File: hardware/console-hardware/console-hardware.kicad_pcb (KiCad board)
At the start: 2 copper layers, 45.7 x 64.8 mm, 42 parts, among them J1 USB_B_Micro, J2 LiPo battery, J3 Conn_01x04, J4 ICSP, J5 Conn_01x20, SW1 SW_Push, SW2 SW_Push, SW3 SW_Push, SW4 SW_Push, SW5 SW_Push, SW6 SW_Push, U1 ATmega32U4-A, U2 MCP73831-2-OT, U3 MIC5219-3.3YM5, X1 16 MHz

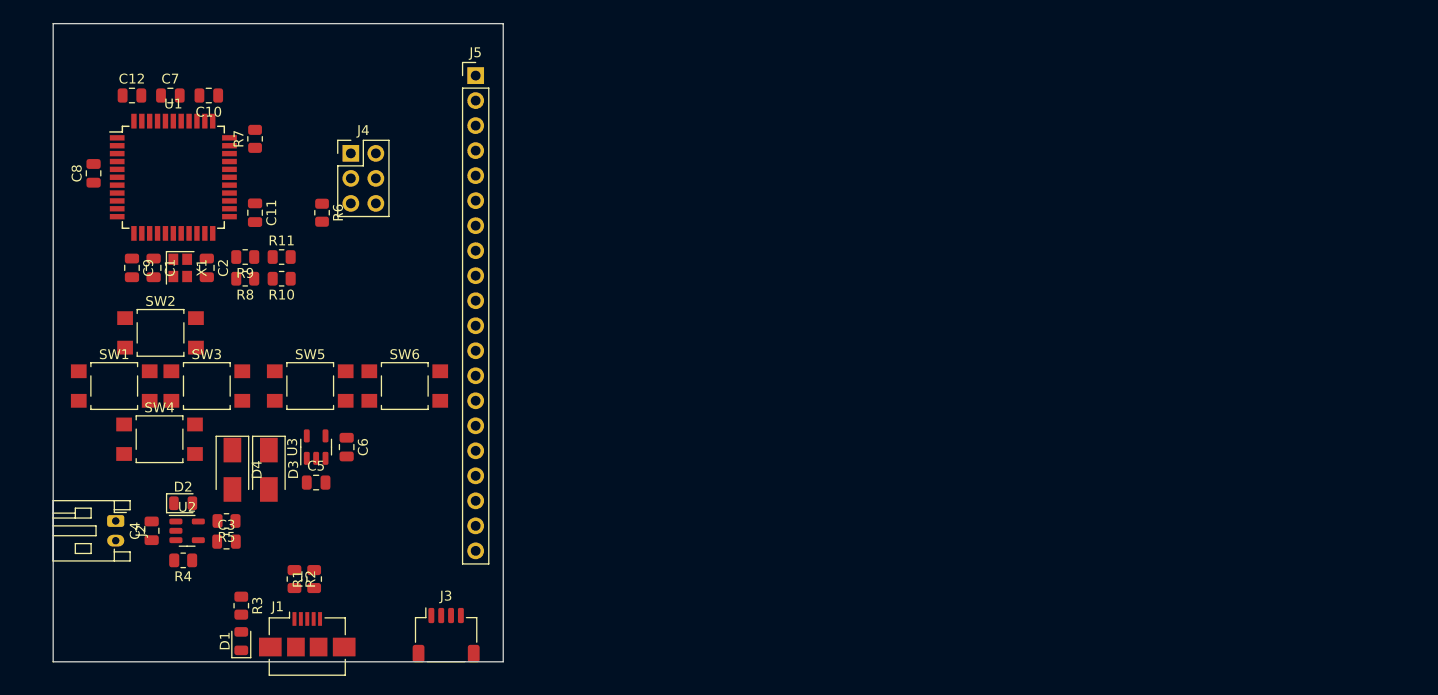
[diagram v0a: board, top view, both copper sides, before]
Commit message: Updated schematic and layout. Added BOM
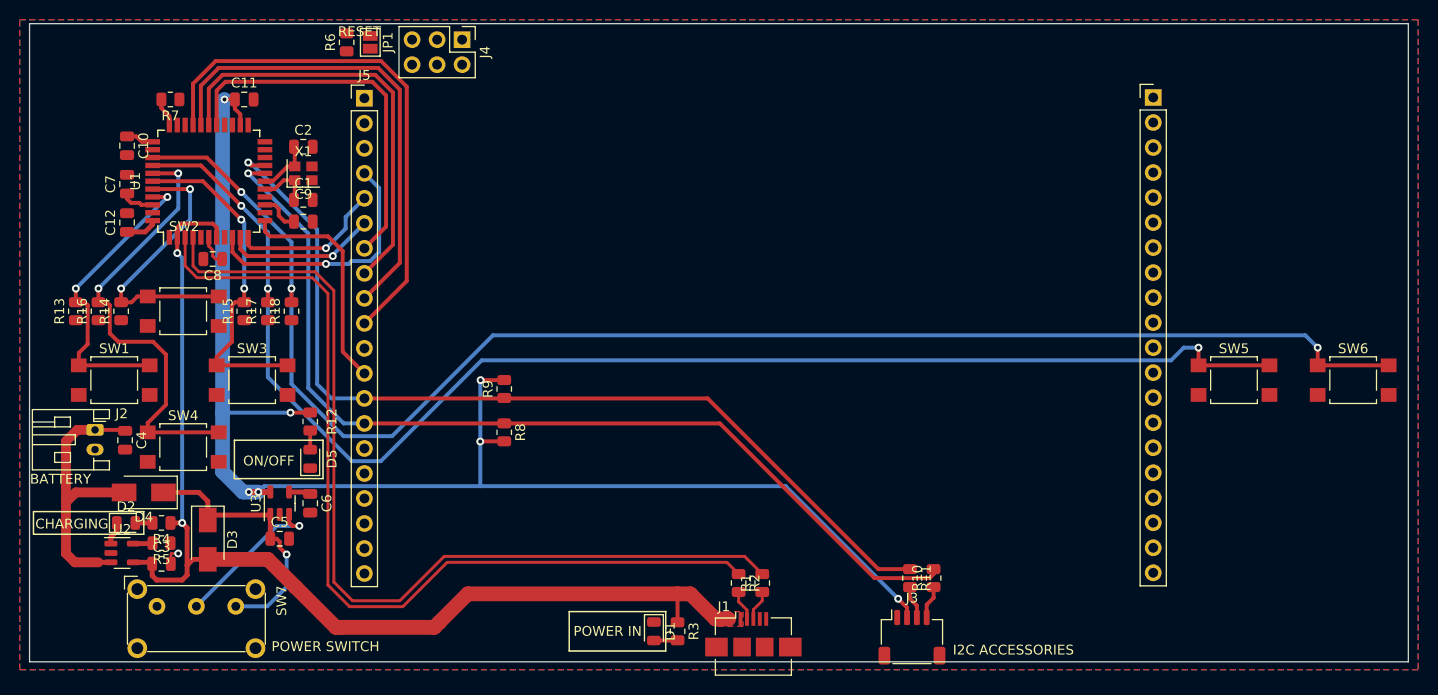
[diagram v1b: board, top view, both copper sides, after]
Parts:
- added D5: Green, LED_SMD:LED_0805_2012Metric, F.Cu at (108.5, 100.6)
- added JP1: Jumper_2_Open, Jumper:SolderJumper-2_P1.3mm_Open_Pad1.0x1.5mm, F.Cu at (114.6, 58.3)
- added R12: 4.7k, Resistor_SMD:R_0805_2012Metric, F.Cu at (108.5, 96.8)
- added R13: 10k, Resistor_SMD:R_0805_2012Metric, F.Cu at (84.7, 85.6)
- added R14: 10k, Resistor_SMD:R_0805_2012Metric, F.Cu at (89.3, 85.6)
- added R15: 10k, Resistor_SMD:R_0805_2012Metric, F.Cu at (101.8, 85.6)
- added R16: 10k, Resistor_SMD:R_0805_2012Metric, F.Cu at (87.0, 85.6)
- added R17: 10k, Resistor_SMD:R_0805_2012Metric, F.Cu at (104.2, 85.6)
- added R18: 10k, Resistor_SMD:R_0805_2012Metric, F.Cu at (106.6, 85.6)
- added REF**: PinHeader_1x20_P2.54mm_Vertical, Connector_PinHeader_2.54mm:PinHeader_1x20_P2.54mm_Vertical, F.Cu at (194.1, 63.9)
- added SW7: SW_SPDT, Button_Switch_THT:SW_E-Switch_EG1224_SPDT_Angled, F.Cu at (92.9, 115.6)
- R3, R4: value 1k -> 4.7k
- moved SW6 96.3 mm to (214.4, 92.6)
- moved SW5 93.8 mm to (202.3, 92.6)
- moved R10 72.8 mm to (171.8, 112.7), turned to 90 degrees
- moved R11 71.6 mm to (169.4, 112.7), turned to -90 degrees
- moved J3 47.3 mm to (169.6, 118.7)
- moved R1 45.5 mm to (154.4, 113.2)
- moved J1 45.3 mm to (153.5, 118.4)
- moved R2 45.1 mm to (152.0, 113.2)
- moved R3 44.4 mm to (145.8, 118.1)
- moved D1 41.9 mm to (143.4, 118.1), turned to -90 degrees
- moved R8 30.6 mm to (128.2, 97.9), turned to -90 degrees
- moved R9 29.5 mm to (128.2, 93.5), turned to 90 degrees
- moved C9 18.0 mm to (107.8, 76.5), turned to 0 degrees
- moved R6 17.5 mm to (112.2, 58.3), turned to 90 degrees
- moved C1 16.7 mm to (107.8, 74.3), turned to 0 degrees
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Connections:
- net Net-(J3-Pad3) renamed /SDA_OUT
- net Net-(J3-Pad4) renamed /SCL_OUT
- J5 pad 1: unconnected-(J5-Pad1) -> +3.3V
- J5 pad 10: unconnected-(J5-Pad10) -> /DISPLAY_LITE
- J5 pad 11: unconnected-(J5-Pad11) -> GND
- J5 pad 12: unconnected-(J5-Pad12) -> /DISPLAY_IRQ
- J5 pad 13: unconnected-(J5-Pad13) -> /SDA
- J5 pad 14: unconnected-(J5-Pad14) -> /SCL
- J5 pad 2: unconnected-(J5-Pad2) -> GND
- J5 pad 3: +3.3V -> /3VO
- J5 pad 4: GND -> /SCK
- J5 pad 5: unconnected-(J5-Pad5) -> /MISO
- J5 pad 6: unconnected-(J5-Pad6) -> /MOSI
- J5 pad 7: unconnected-(J5-Pad7) -> /DISPLAY_CS
- J5 pad 8: unconnected-(J5-Pad8) -> /DISPLAY_DC
- J5 pad 9: unconnected-(J5-Pad9) -> /DISPLAY_RST
- U1 pad 12: unconnected-(U1-Pad12) -> /DISPLAY_IRQ
- U1 pad 27: unconnected-(U1-Pad27) -> /DISPLAY_CS
- U1 pad 28: unconnected-(U1-Pad28) -> /DISPLAY_DC
- U1 pad 29: unconnected-(U1-Pad29) -> /DISPLAY_RST
- U1 pad 30: unconnected-(U1-Pad30) -> /DISPLAY_LITE
- U3 pad 3: unconnected-(U3-Pad3) -> /ON/~{OFF}
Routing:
- net +3.3V: track 0.00 -> 155.4 mm, vias 0 -> 7
- net Net-(R18-Pad2): track 0.00 -> 153.6 mm, vias 0 -> 3
- net Net-(R17-Pad2): track 0.00 -> 142.4 mm, vias 0 -> 3
- net VBUS: track 0.00 -> 112.8 mm, vias 0 -> 2
- net /SCL: track 0.00 -> 98.2 mm, vias 0 -> 1
- net /SDA: track 0.00 -> 95.3 mm, vias 0 -> 1
- net /RD+: track 0.00 -> 94.7 mm
- net /RD-: track 0.00 -> 93.1 mm
- net /DISPLAY_LITE: track 0.00 -> 53.7 mm
- net /DISPLAY_RST: track 0.00 -> 48.5 mm
- net Net-(R16-Pad2): track 0.00 -> 45.6 mm, vias 0 -> 2
- net /DISPLAY_DC: track 0.00 -> 43.3 mm
- net /DISPLAY_CS: track 0.00 -> 38.1 mm
- net Net-(R15-Pad2): track 0.00 -> 34.4 mm, vias 0 -> 2
- net Net-(R13-Pad2): track 0.00 -> 31.0 mm, vias 0 -> 2
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- added copper zone on B.Cu, net GND
- added copper zone on F.Cu, net GND
- added copper zone on F.Cu, net VBUS
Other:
- board size 45.7 x 64.8 mm -> 140 x 64.8 mm
- board text added: "BATTERY"
- board text added: "CHARGING"
- board text added: "I2C ACCESSORIES"
- board text added: "ON/OFF"
- board text added: "POWER IN"
- board text added: "POWER SWITCH"
- board text added: "RESET"
